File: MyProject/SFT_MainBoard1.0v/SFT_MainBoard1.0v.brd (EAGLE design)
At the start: 100 x 65 mm, 44 parts, among them CON1 I2C1, CON2 I2C1, CON3 I2C1, CON4 I2C1, CON5 I2C2, CON6 I2C2, CON7 I2C2, CON8 I2C2, CON9 B4B-ZR, M1 SBDBT

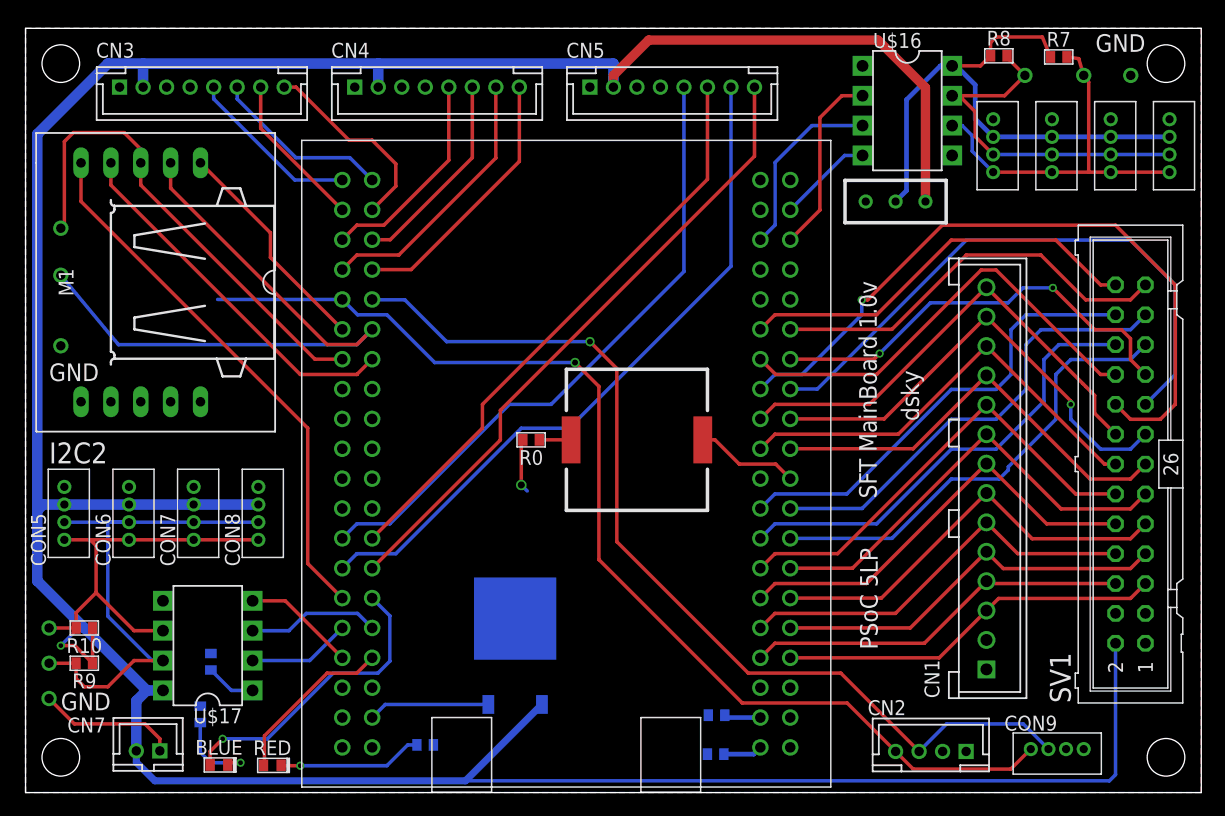
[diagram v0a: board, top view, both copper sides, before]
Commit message: kyuukei reset
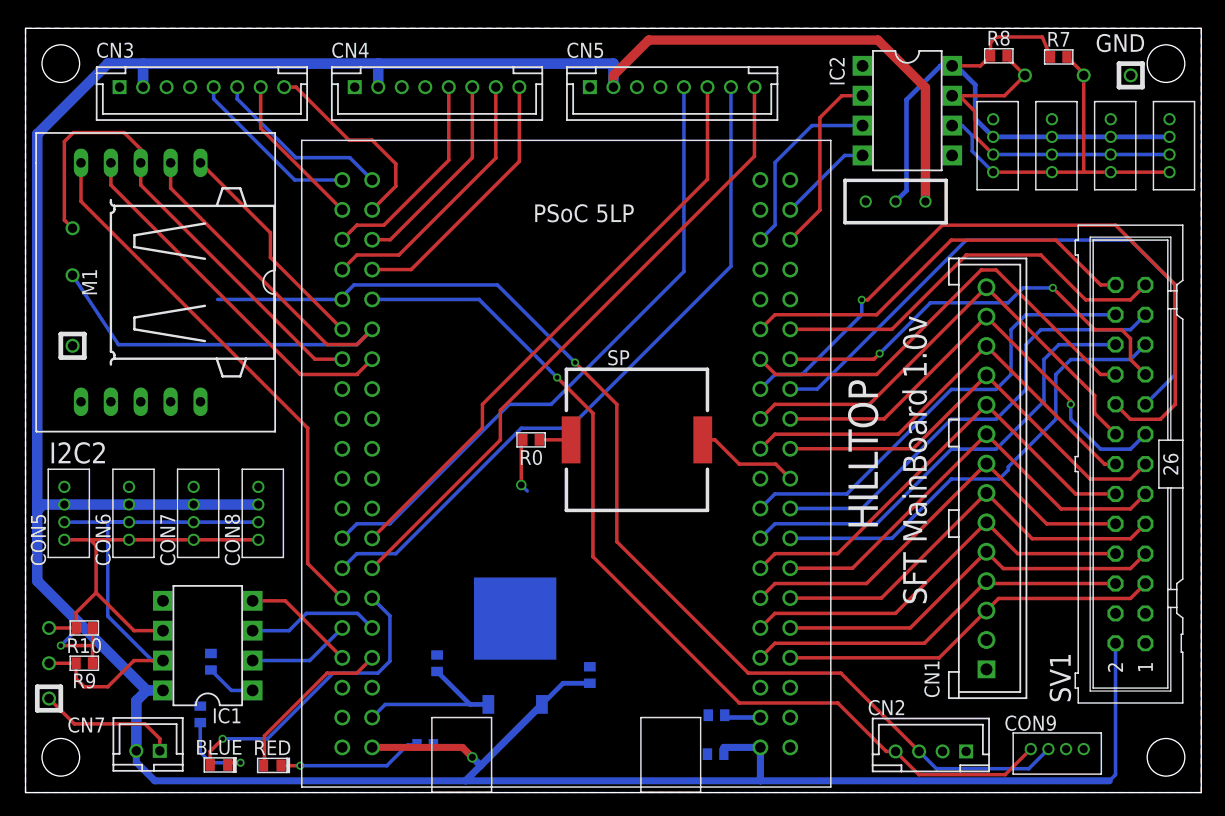
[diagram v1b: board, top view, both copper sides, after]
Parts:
- added C4, C5: (no value), 02_C:1608
- moved U$38 1.00 mm to (4.00, 38.0)
- moved U$82 1.00 mm to (4.00, 44.0)
- moved U$83 1.00 mm to (4.00, 48.0)
- renumbered U$16 to IC2, U$17 to IC1, U$41 to SP
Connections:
- removed net V_DDIN: C3.P$1, U$2.P$2
- removed net V_DDIN2: U$2.P$41
- net +3.3V: now also C5.P$1
- net +5V: now also C3.P$1, C4.P$1, U$2.P$2, U$2.P$41
- net GND: now also C4.P$2, C5.P$2
- net P12_4: now also CN2.3, CON9.3; no longer CN2.4, CON9.4
- net P12_5: now also CN2.4, CON9.4; no longer CN2.3, CON9.3
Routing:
- net +5V: track 289.1 -> 309.7 mm, vias 1 -> 2
- net +3.3V: track 17.7 -> 23.2 mm
- net V_DDIN: track 3.34 -> 0.00 mm
- net P12_5: track 83.9 -> 80.9 mm
- net P12_4: track 95.0 -> 95.9 mm
- net P6_5: track 55.1 -> 54.5 mm
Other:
- board text added: "HILLTOP"
- board text removed: "dsky"

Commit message: tetuya
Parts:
- added DRILEGEND: (no value), drilegend:DRILEGEND
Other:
- board text added: "穴図"

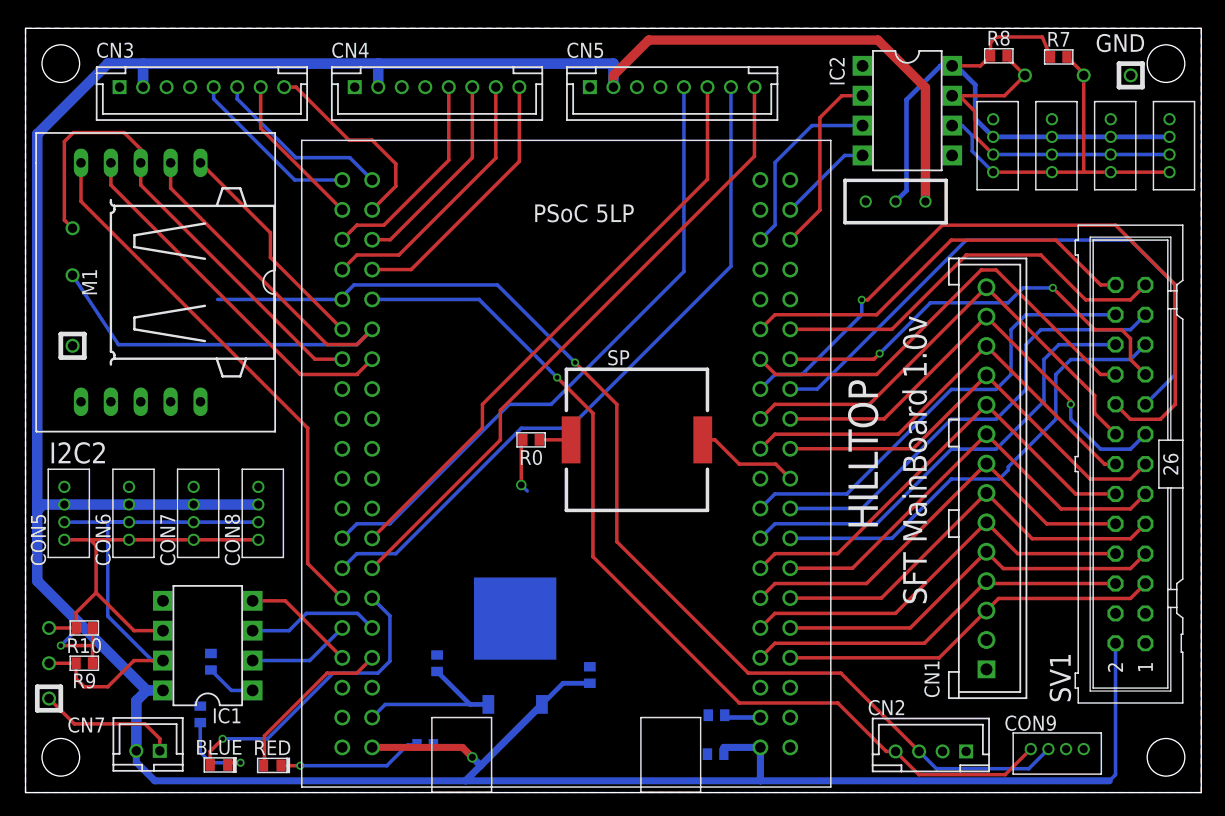
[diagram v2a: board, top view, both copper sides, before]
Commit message: test2
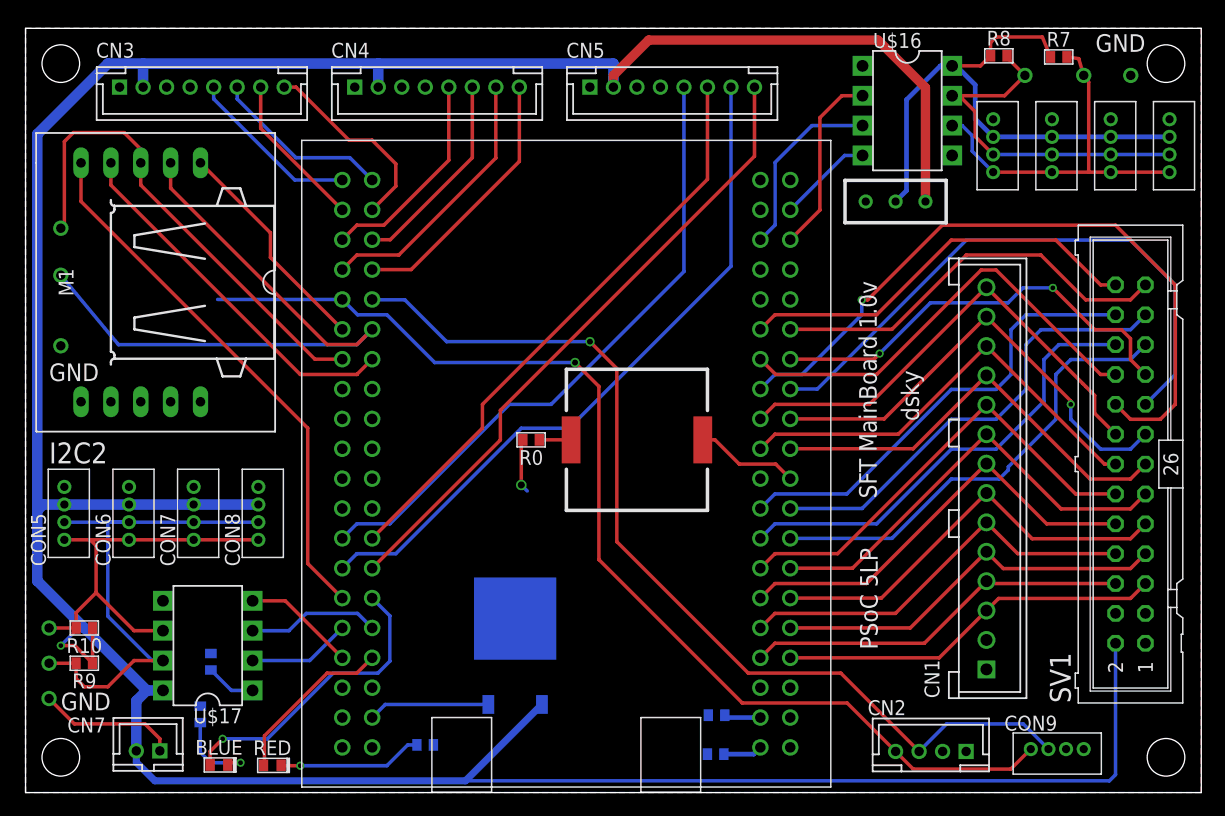
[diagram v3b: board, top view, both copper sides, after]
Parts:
- removed C4, C5: (no value), 02_C:1608
- removed DRILEGEND: (no value), drilegend:DRILEGEND
- moved U$38 1.00 mm to (3.00, 38.0)
- moved U$82 1.00 mm to (3.00, 44.0)
- moved U$83 1.00 mm to (3.00, 48.0)
- renumbered IC1 to U$17, IC2 to U$16, SP to U$41
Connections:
- new net V_DDIN: C3.P$1, U$2.P$2
- new net V_DDIN2: U$2.P$41
- net +3.3V: no longer C5.P$1
- net +5V: no longer C3.P$1, C4.P$1, U$2.P$2, U$2.P$41
- net GND: no longer C4.P$2, C5.P$2
- net P12_4: now also CN2.4, CON9.4; no longer CN2.3, CON9.3
- net P12_5: now also CN2.3, CON9.3; no longer CN2.4, CON9.4
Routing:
- net +5V: track 309.7 -> 289.1 mm, vias 2 -> 1
- net +3.3V: track 23.2 -> 17.7 mm
- net V_DDIN: track 0.00 -> 3.34 mm
- net P12_5: track 80.9 -> 83.9 mm
- net P12_4: track 95.9 -> 95.0 mm
- net P6_5: track 54.5 -> 55.1 mm
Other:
- board text added: "dsky"
- board text removed: "HILLTOP"
- board text removed: "穴図"
